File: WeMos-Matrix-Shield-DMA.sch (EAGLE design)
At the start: 21 parts, among them J3 TWIG-2.0-DIP, U1 LDR, X1 5202-02-N-02

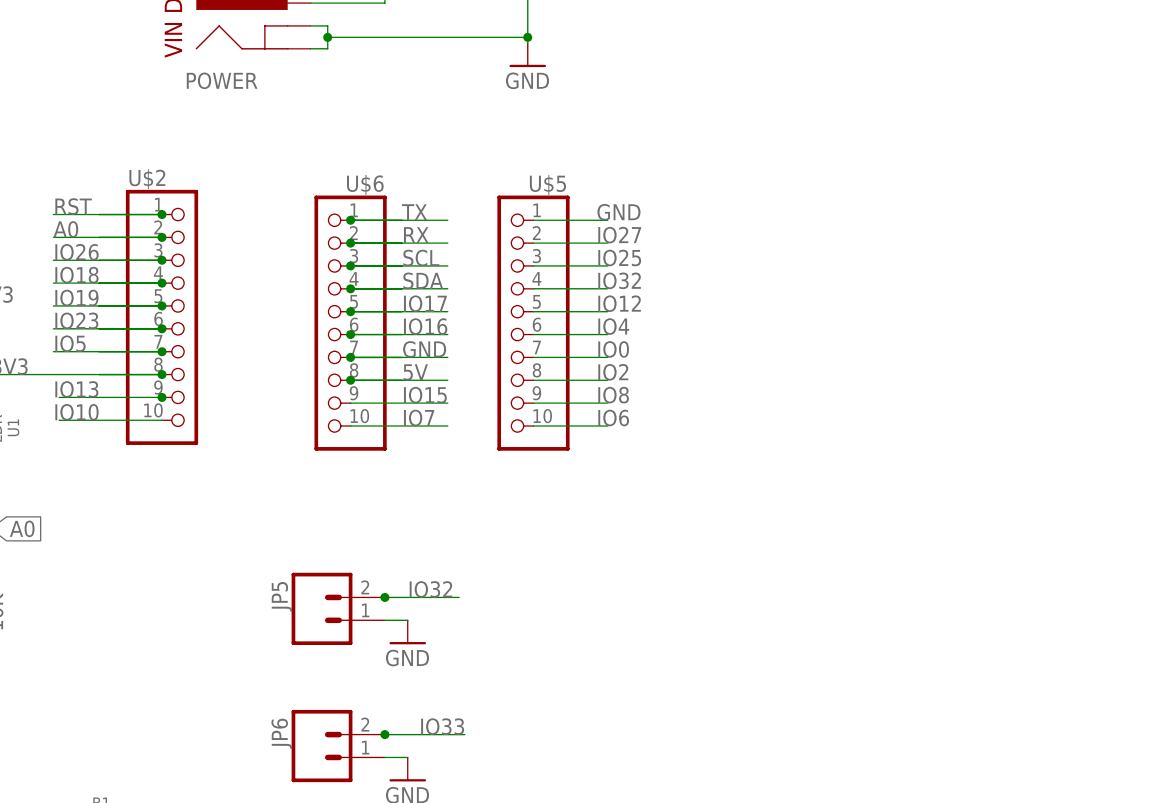
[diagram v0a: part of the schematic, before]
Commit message: bump to v1.8a
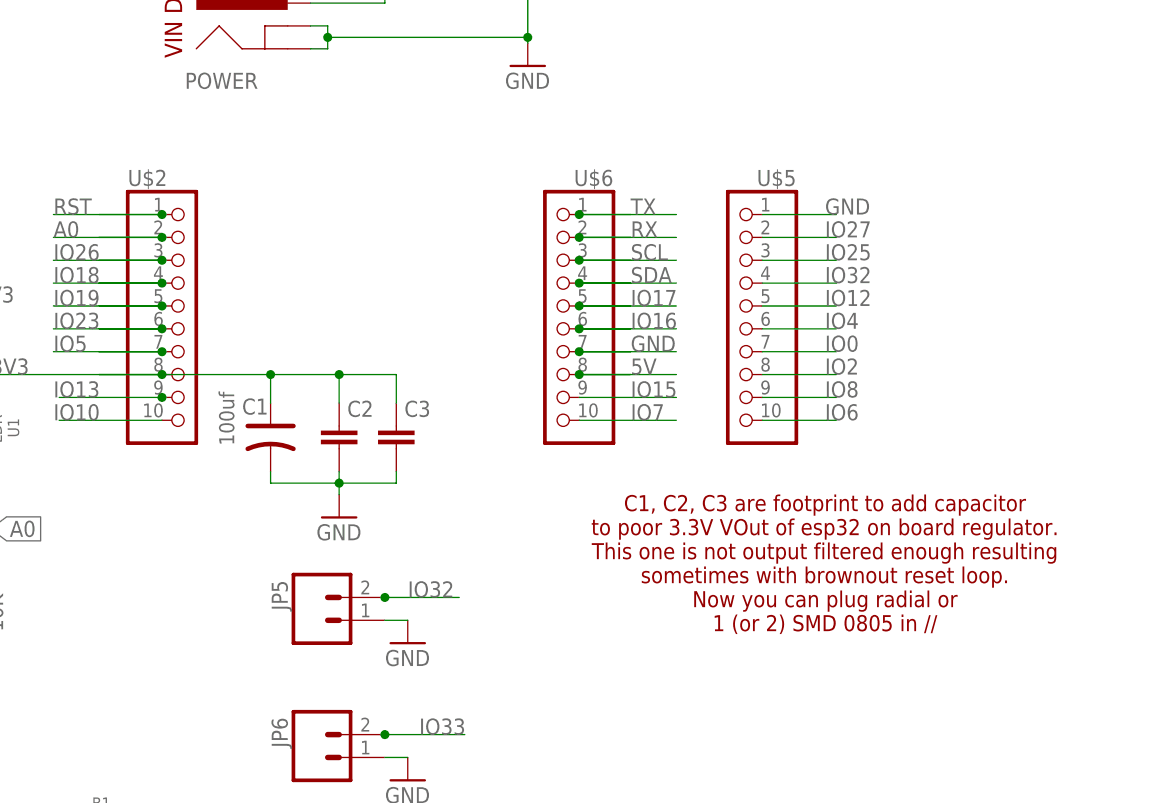
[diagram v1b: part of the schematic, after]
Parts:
- added C1: 100uf, Seeed-Capacitor:DIP-ALUMINUM-47UF-16V(D5-H7MM)
- added C2, C3: (no value), _c2h:CAP0805-CAP-LARGEPADS
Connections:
- net 3V3: now also C1.+, C2.1, C3.1
- net GND: now also C1.-, C2.2, C3.2
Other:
- note added: "C1, C2, C3 are footprint to add capacitor to poor 3.3V VOut of esp32 on board regulator. This one is not output filtered enough resulting sometimes with brownout reset loop. Now you can plug radial or 1 (or 2) SMD 0805 in //"
- moved on the sheet: U$5, U$6
